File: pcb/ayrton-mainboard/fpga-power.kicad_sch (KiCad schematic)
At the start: 1 part, among them U2 XC7K160T-2FFG676C

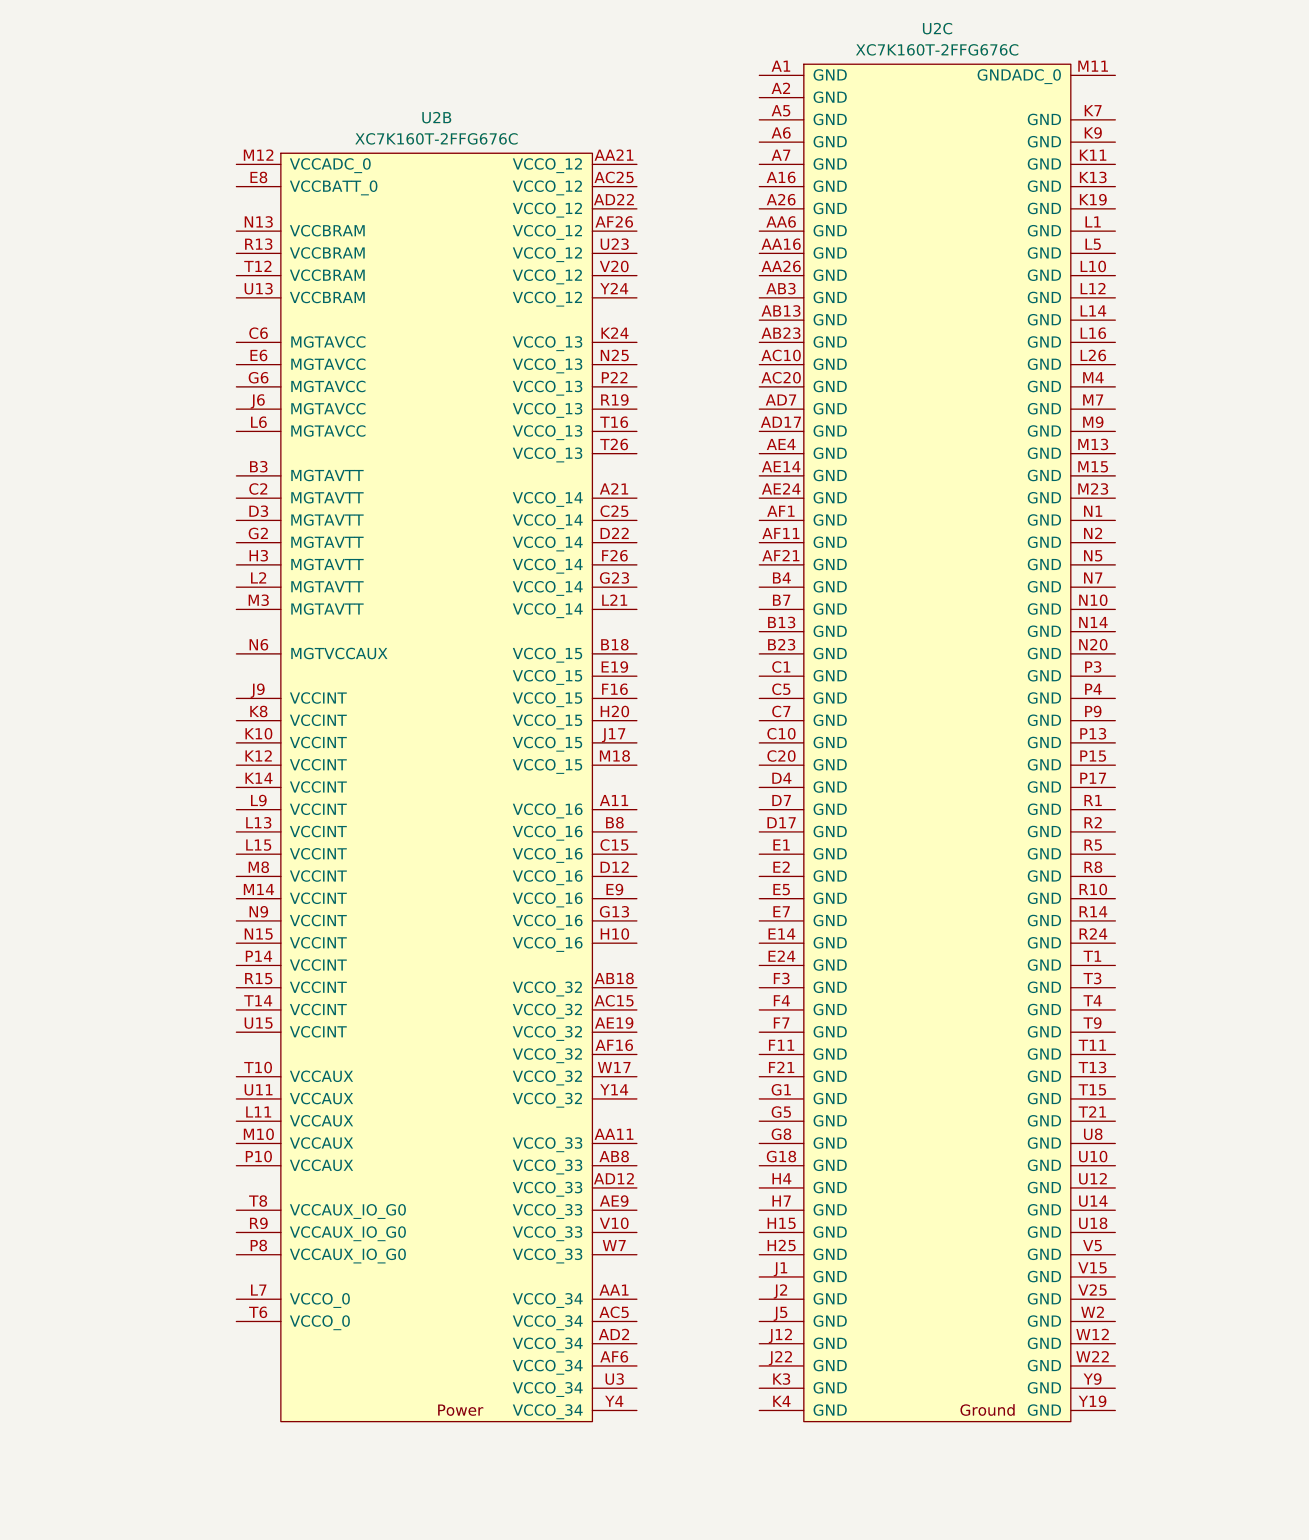
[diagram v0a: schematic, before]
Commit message: Continued initial system design
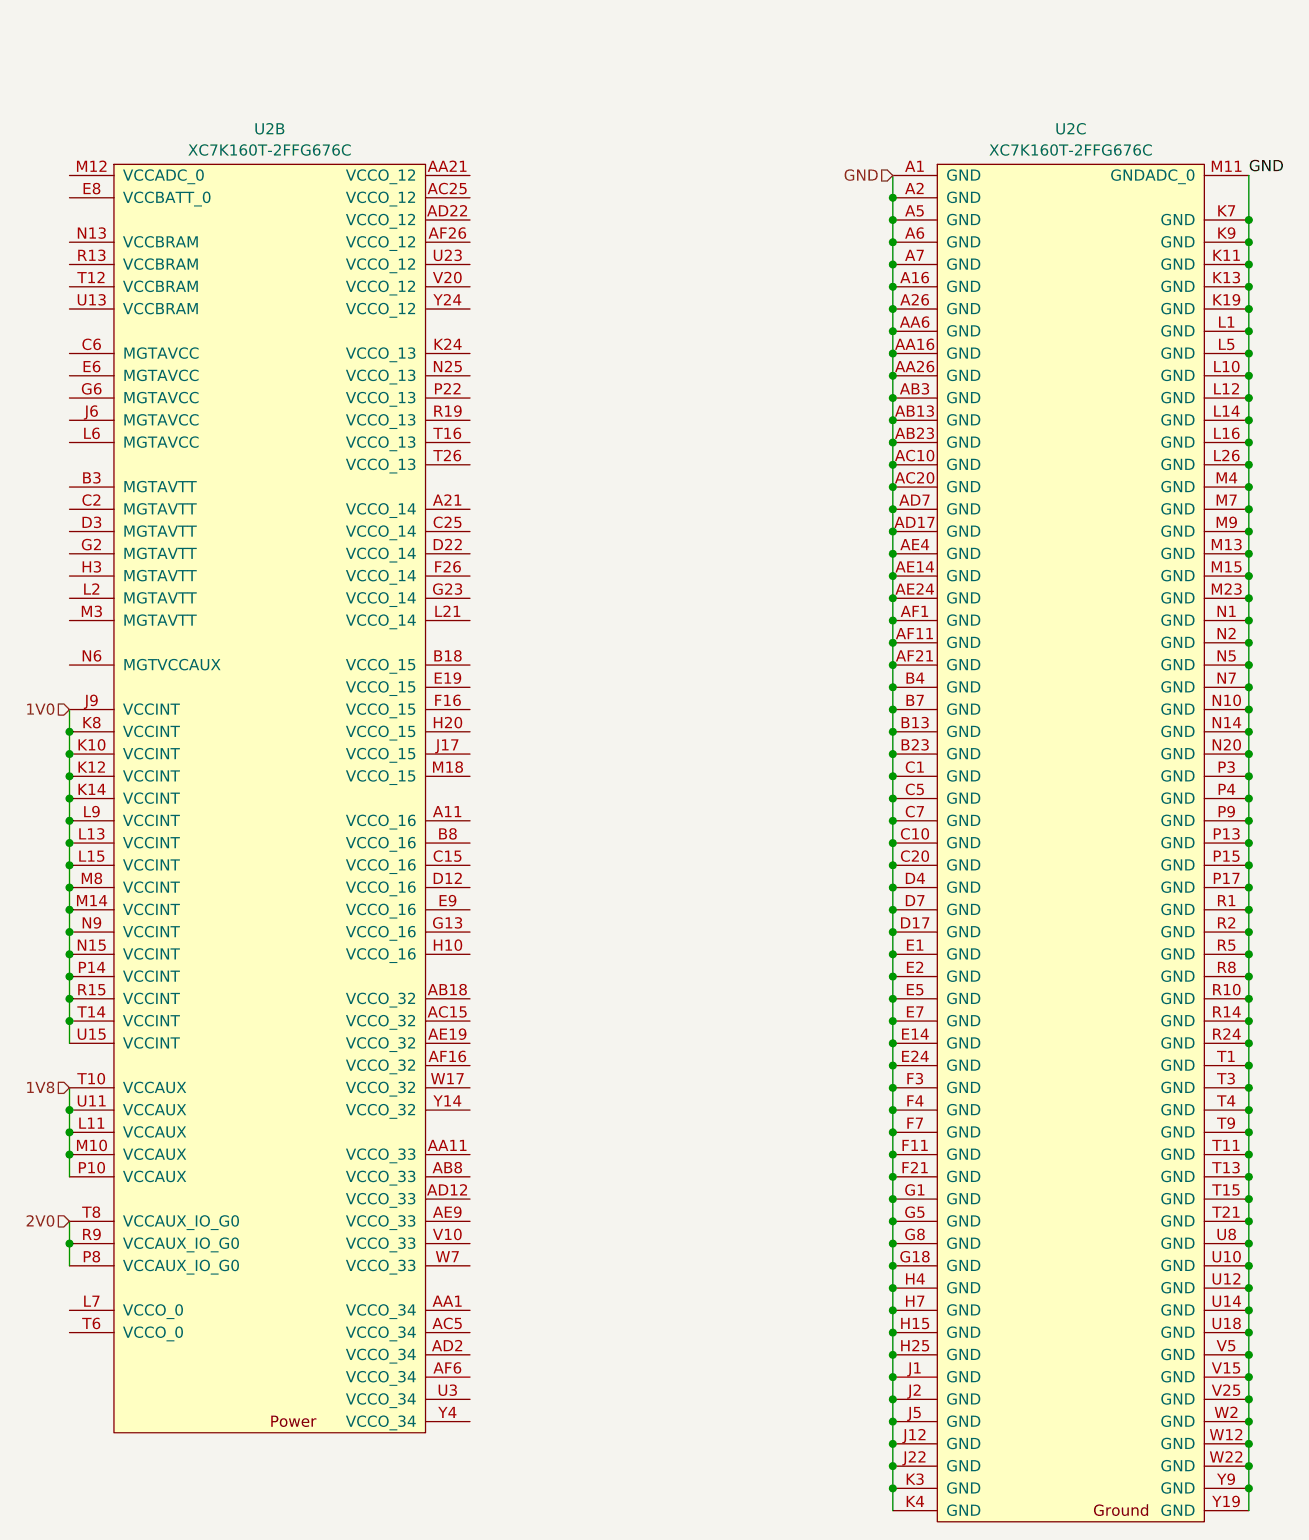
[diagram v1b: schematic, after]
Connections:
- net GND: now reaches U2.A1 (GND)
- net GND: now also U2.A16 (GND), U2.A2 (GND), U2.A26 (GND), U2.A5 (GND), U2.A6 (GND), U2.A7 (GND), U2.AA16 (GND), U2.AA26 (GND), U2.AA6 (GND), U2.AB13 (GND), U2.AB23 (GND), U2.AB3 (GND), U2.AC10 (GND), U2.AC20 (GND), U2.AD17 (GND), U2.AD7 (GND), U2.AE14 (GND), U2.AE24 (GND), U2.AE4 (GND), U2.AF1 (GND), U2.AF11 (GND), U2.AF21 (GND), U2.B13 (GND), U2.B23 (GND), U2.B4 (GND), U2.B7 (GND), U2.C1 (GND), U2.C10 (GND), U2.C20 (GND), U2.C5 (GND), U2.C7 (GND), U2.D17 (GND), U2.D4 (GND), U2.D7 (GND), U2.E1 (GND), U2.E14 (GND), U2.E2 (GND), U2.E24 (GND), U2.E5 (GND), U2.E7 (GND), U2.F11 (GND), U2.F21 (GND), U2.F3 (GND), U2.F4 (GND), U2.F7 (GND), U2.G1 (GND), U2.G18 (GND), U2.G5 (GND), U2.G8 (GND), U2.H15 (GND), U2.H25 (GND), U2.H4 (GND), U2.H7 (GND), U2.J1 (GND), U2.J12 (GND), U2.J2 (GND), U2.J22 (GND), U2.J5 (GND), U2.K11 (GND), U2.K13 (GND), U2.K19 (GND), U2.K3 (GND), U2.K4 (GND), U2.K7 (GND), U2.K9 (GND), U2.L1 (GND), U2.L10 (GND), U2.L12 (GND), U2.L14 (GND), U2.L16 (GND), U2.L26 (GND), U2.L5 (GND), U2.M11 (GNDADC_0), U2.M13 (GND), U2.M15 (GND), U2.M23 (GND), U2.M4 (GND), U2.M7 (GND), U2.M9 (GND), U2.N1 (GND), U2.N10 (GND), U2.N14 (GND), U2.N2 (GND), U2.N20 (GND), U2.N5 (GND), U2.N7 (GND), U2.P13 (GND), U2.P15 (GND), U2.P17 (GND), U2.P3 (GND), U2.P4 (GND), U2.P9 (GND), U2.R1 (GND), U2.R10 (GND), U2.R14 (GND), U2.R2 (GND), U2.R24 (GND), U2.R5 (GND), U2.R8 (GND), U2.T1 (GND), U2.T11 (GND), U2.T13 (GND), U2.T15 (GND), U2.T21 (GND), U2.T3 (GND), U2.T4 (GND), U2.T9 (GND), U2.U10 (GND), U2.U12 (GND), U2.U14 (GND), U2.U18 (GND), U2.U8 (GND), U2.V15 (GND), U2.V25 (GND), U2.V5 (GND), U2.W12 (GND), U2.W2 (GND), U2.W22 (GND), U2.Y19 (GND), U2.Y9 (GND)
- net 1V0: now reaches U2.J9 (VCCINT)
- net 1V0: now also U2.K10 (VCCINT), U2.K12 (VCCINT), U2.K14 (VCCINT), U2.K8 (VCCINT), U2.L13 (VCCINT), U2.L15 (VCCINT), U2.L9 (VCCINT), U2.M14 (VCCINT), U2.M8 (VCCINT), U2.N15 (VCCINT), U2.N9 (VCCINT), U2.P14 (VCCINT), U2.R15 (VCCINT), U2.T14 (VCCINT), U2.U15 (VCCINT)
- net 1V8: now reaches U2.L11 (VCCAUX)
- net 1V8: now also U2.M10 (VCCAUX), U2.P10 (VCCAUX), U2.T10 (VCCAUX), U2.U11 (VCCAUX)
- net 2V0: now reaches U2.P8 (VCCAUX_IO_G0)
- net 2V0: now also U2.R9 (VCCAUX_IO_G0), U2.T8 (VCCAUX_IO_G0)
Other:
- moved on the sheet: U2B, U2C
